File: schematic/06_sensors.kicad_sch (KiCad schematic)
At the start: 42 parts, among them J601 HALL, J602 ENCODER, U601 TPS2553DBVR-1, U602 TPS2553DBVR-1, U603 SN74LVC3G17DCTR, U604 SN74LVC3G17DCTR

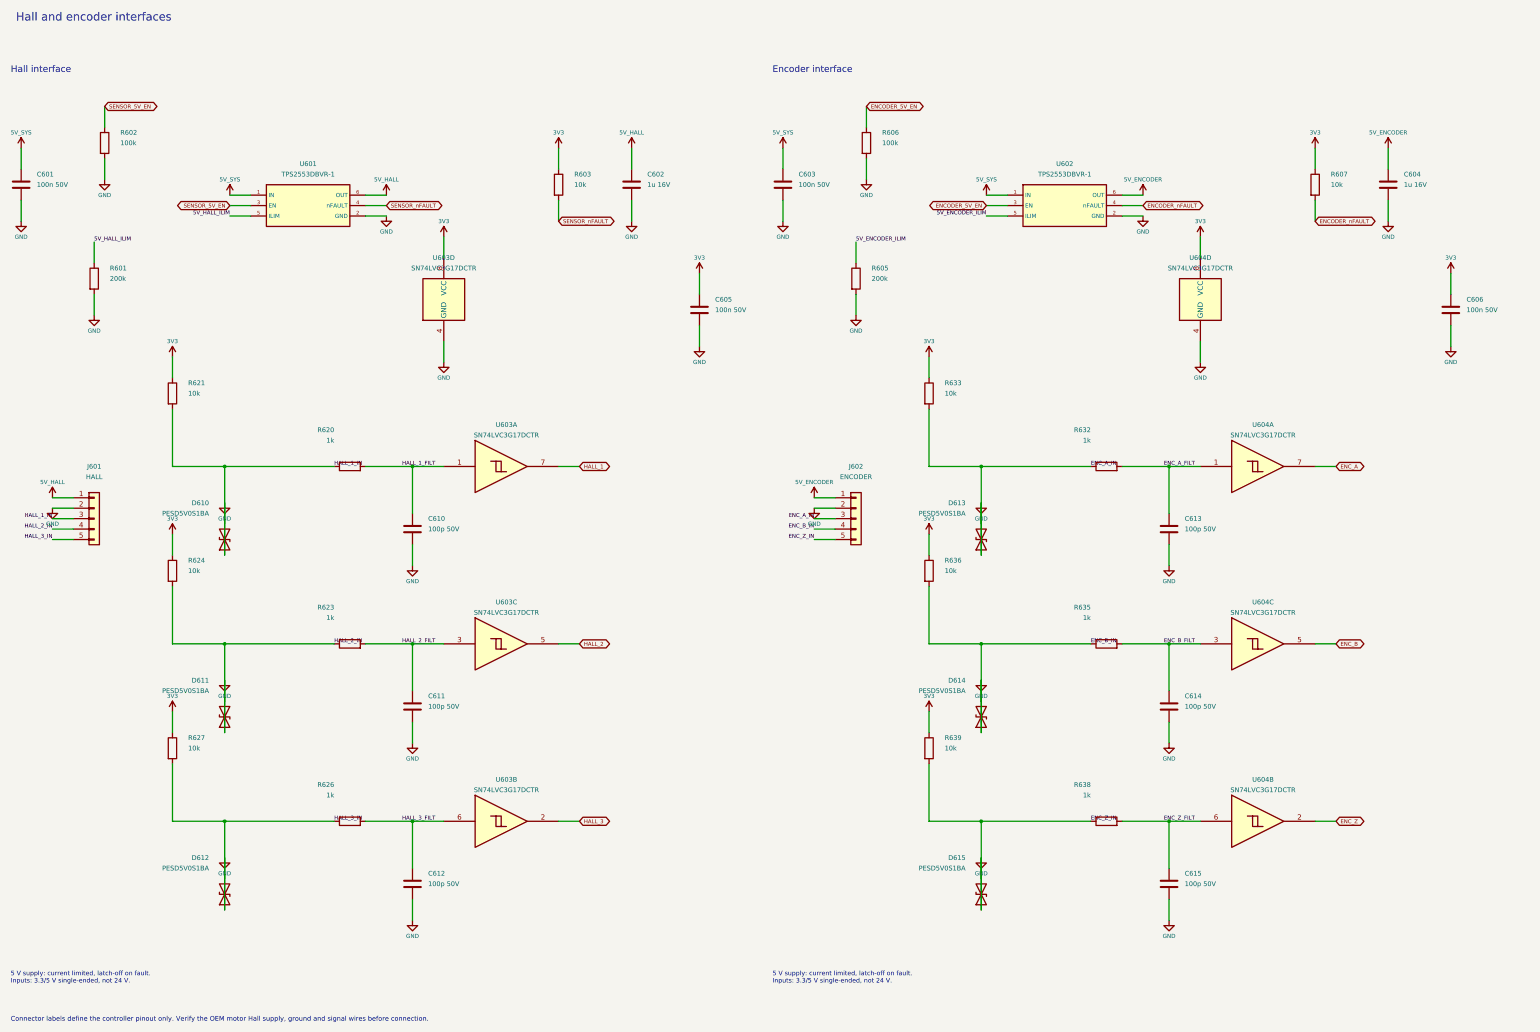
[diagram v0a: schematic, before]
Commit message: devlog 03
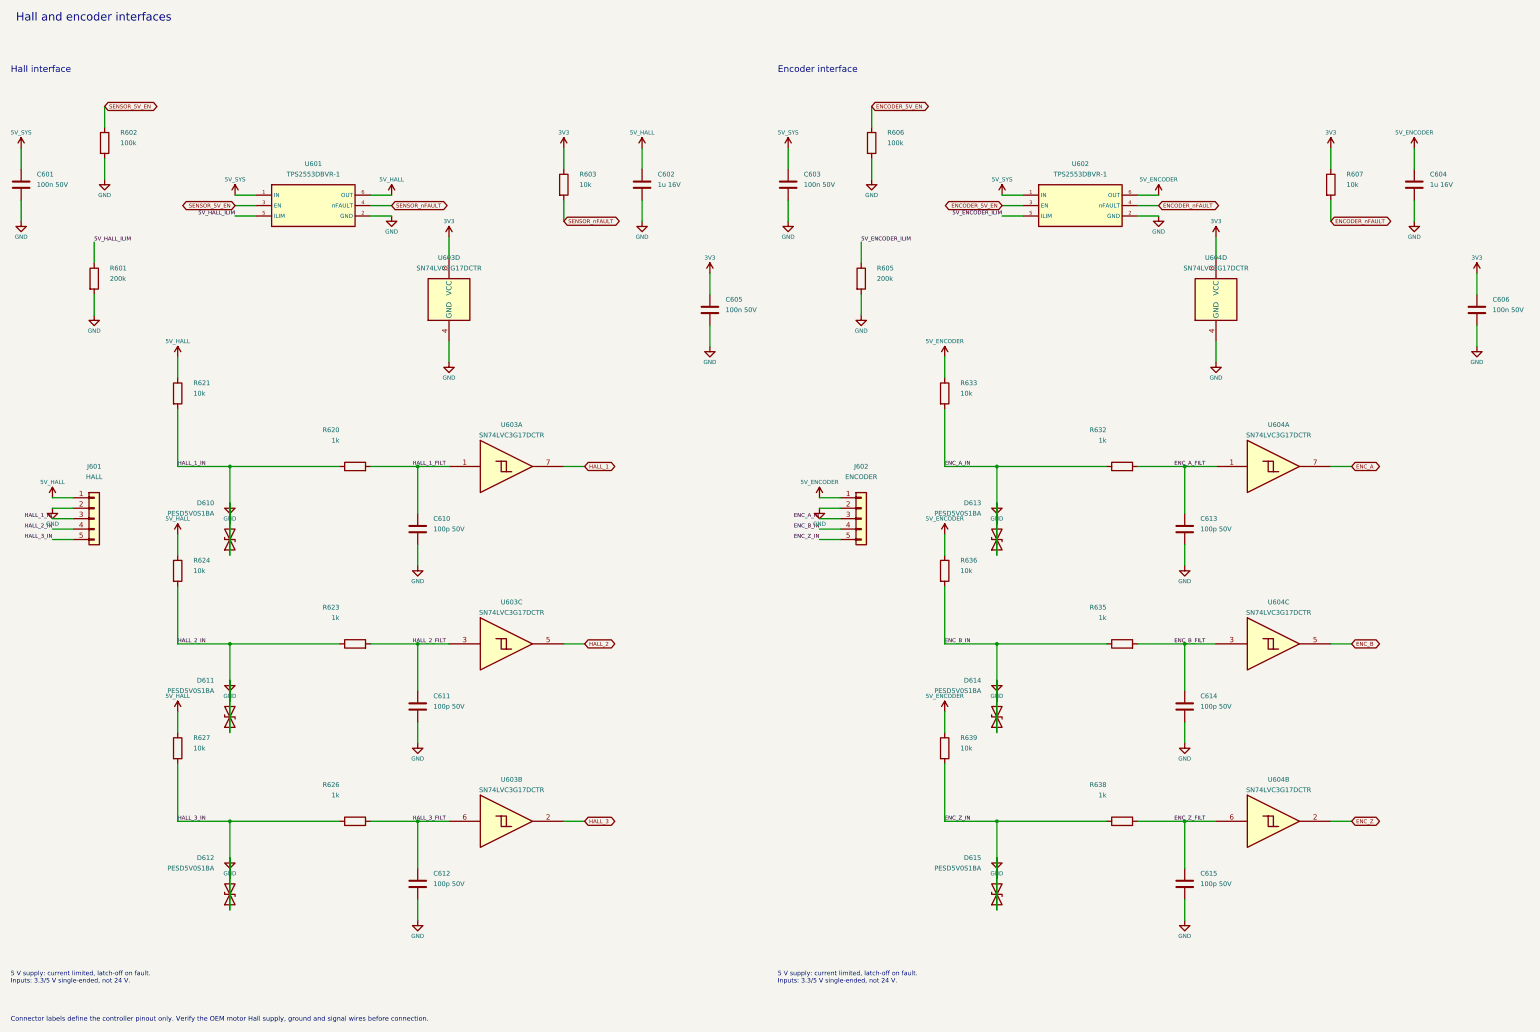
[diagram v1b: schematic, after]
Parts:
- D610, D611, D612, D613, D614, D615: Manufacturer (none) -> Nexperia
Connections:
- net 3V3: no longer R621.1, R624.1, R627.1, R633.1, R636.1, R639.1
- net 5V_ENCODER: now also R633.1, R636.1, R639.1
- net 5V_HALL: now also R621.1, R624.1, R627.1
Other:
- moved on the sheet: C602, C603, C604, C605, C606, C610, C611, C612, C613, C614, C615, D610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
